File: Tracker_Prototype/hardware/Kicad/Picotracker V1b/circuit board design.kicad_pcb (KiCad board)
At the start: 2 copper layers, 47.4 x 20.1 mm, 55 parts, among them IC7 SPV1040, J1 Conn_01x06, J2 GND, J3 +SOL, J4 BATT_V+, J5 BATT_GND, J6 ICSS LOGO, Q1 Q_PMOS_DGS, SW1 SW_Push, U2 TPS62740, U3 CMWX1ZZABZ-078, U4 MAX-M8C, U6 MS5607-02BA

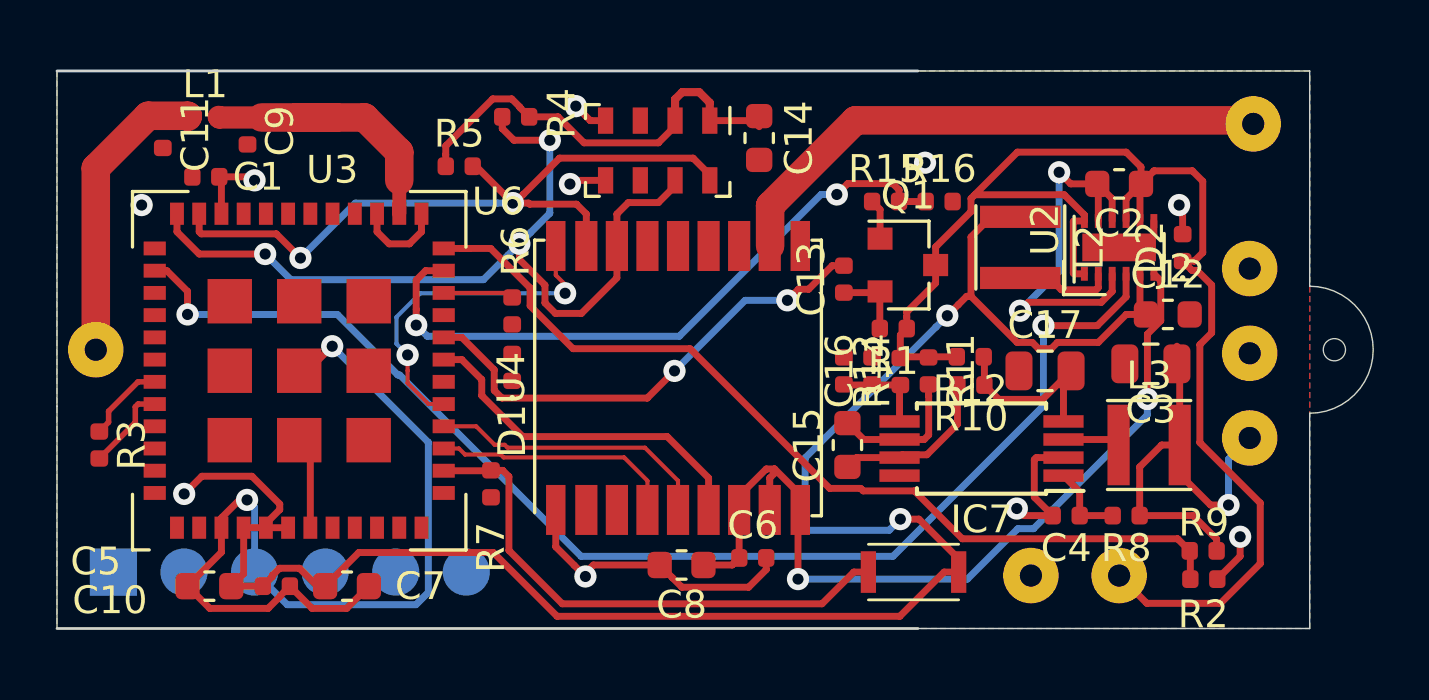
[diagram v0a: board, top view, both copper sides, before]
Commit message: Finished the routing of the b variant.
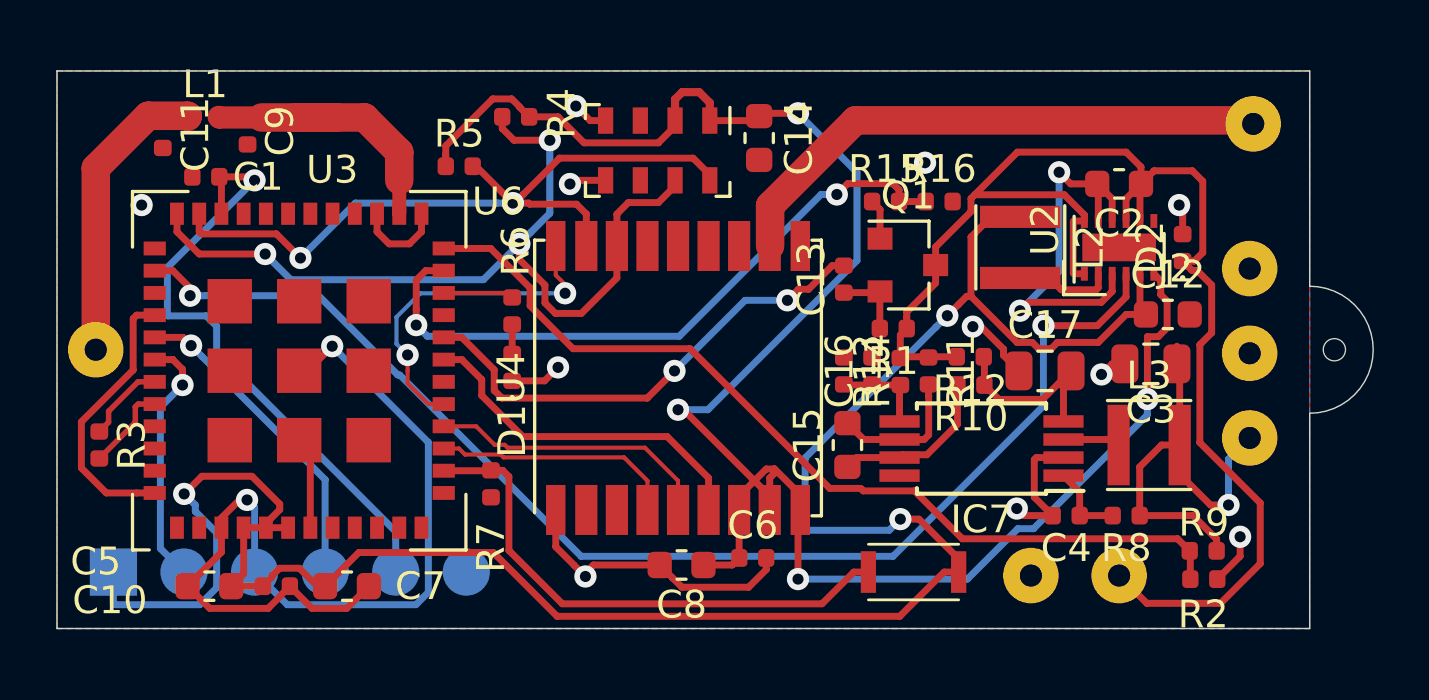
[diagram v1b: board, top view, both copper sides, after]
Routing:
- net SENSOR_VCC: track 47.2 -> 68.7 mm, vias 2 -> 4
- net /RESET: track 2.68 -> 22.3 mm
- net /SWDIO: track 0.09 -> 11.7 mm, vias 0 -> 1
- net /TCXO_EN: track 0.00 -> 9.99 mm
- net /SWCLK: track 0.00 -> 9.12 mm, vias 0 -> 1
- net VCC: track 69.1 -> 78.0 mm
- net GND: track 78.7 -> 84.0 mm, vias 12 -> 15
- net (no net): track 1.94 -> 0.00 mm
- net Net-(D1-Pad2): track 0.00 -> 1.06 mm
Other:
- outline, holes or cut-outs redrawn
